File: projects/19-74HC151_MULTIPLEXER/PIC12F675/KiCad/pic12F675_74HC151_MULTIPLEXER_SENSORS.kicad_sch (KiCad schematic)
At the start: 13 parts, among them M1 Motor_DC, M2 Motor_DC, Q1 NMOS, Q2 NMOS, U1 PIC12F675-IP, U2 74151, U3 LM35-LP, U4 A1369xUA-10, U5 LM35-LP, U6 A1369xUA-10

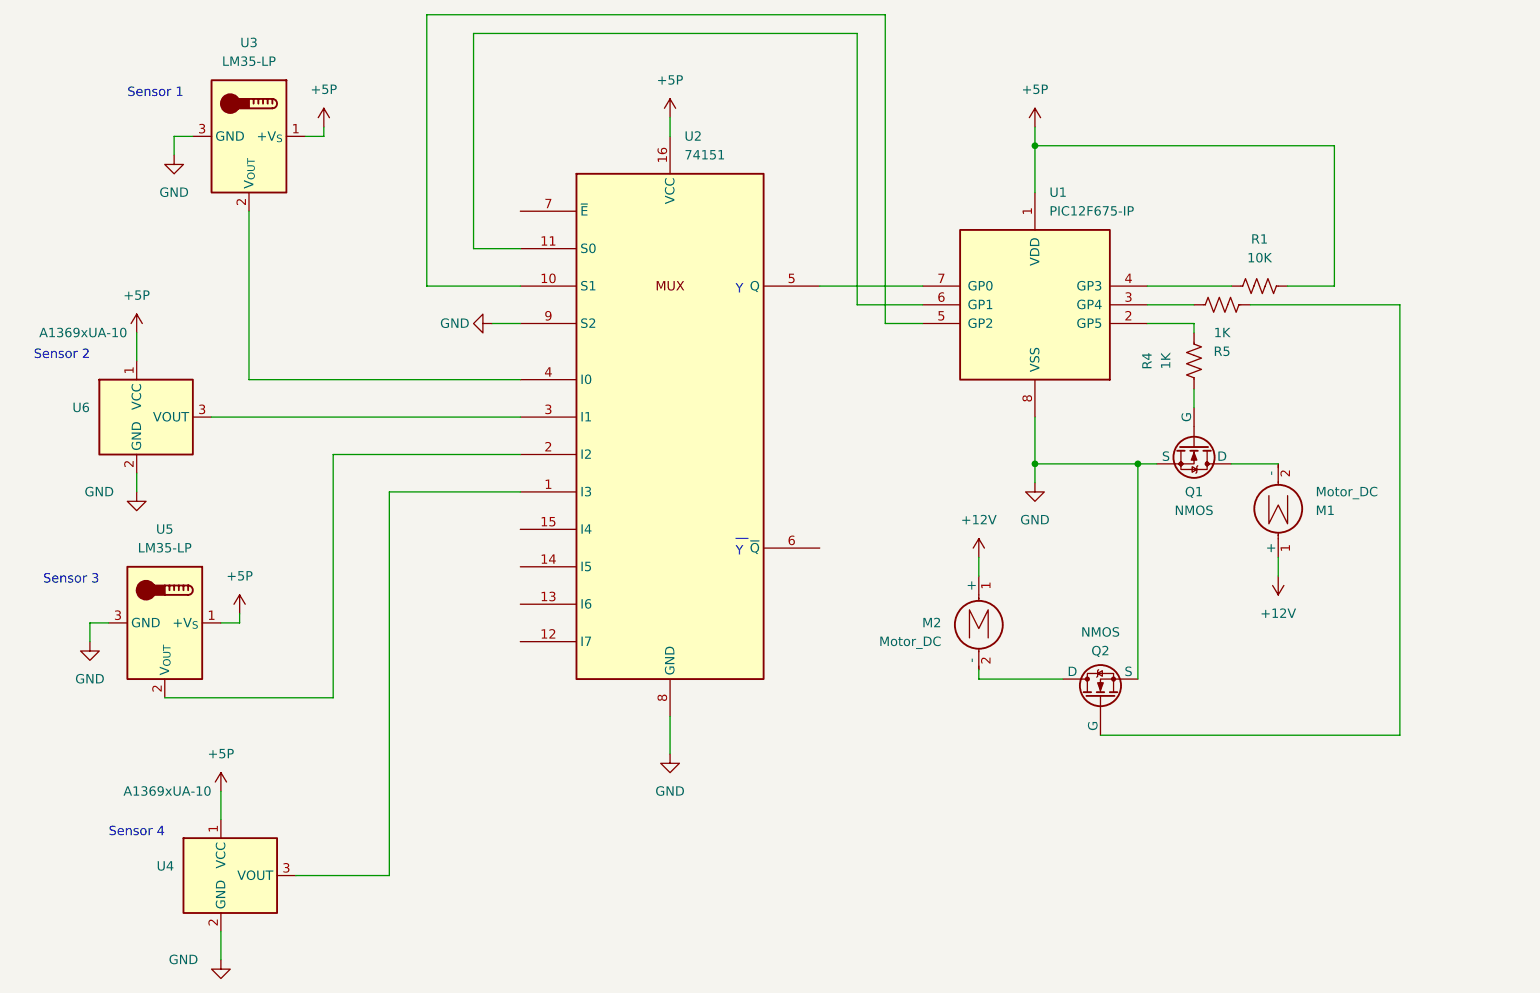
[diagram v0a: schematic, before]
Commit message: Doc
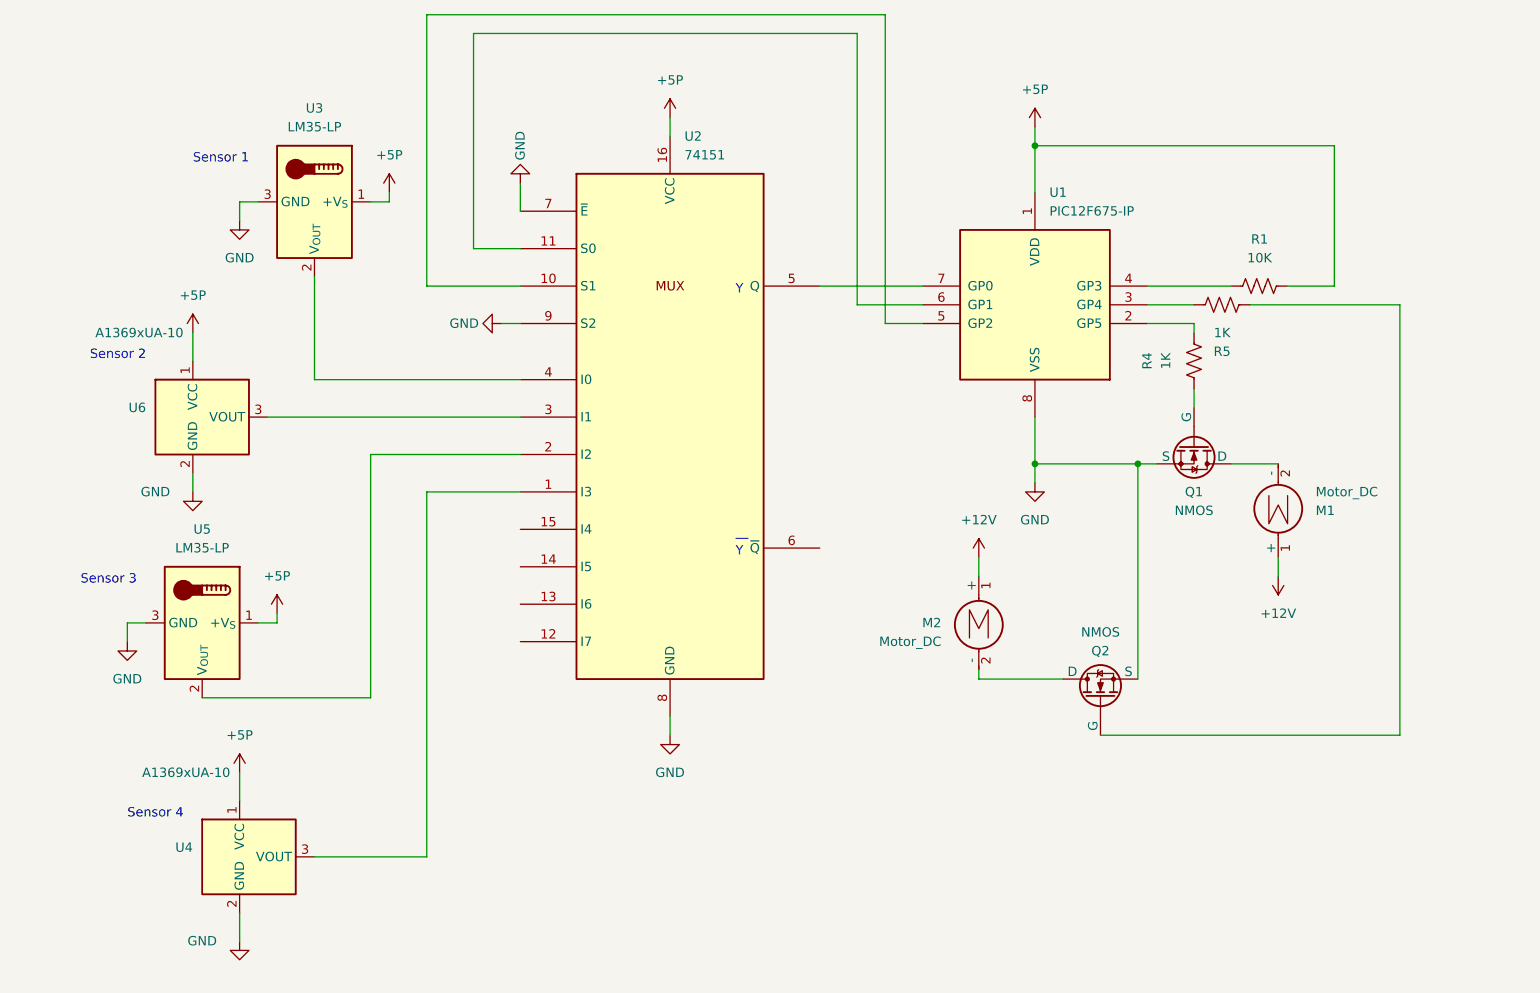
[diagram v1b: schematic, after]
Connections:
- net GND: now also U2.7 (~{E})
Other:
- moved on the sheet: U3, U4, U5, U6

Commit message: Doc
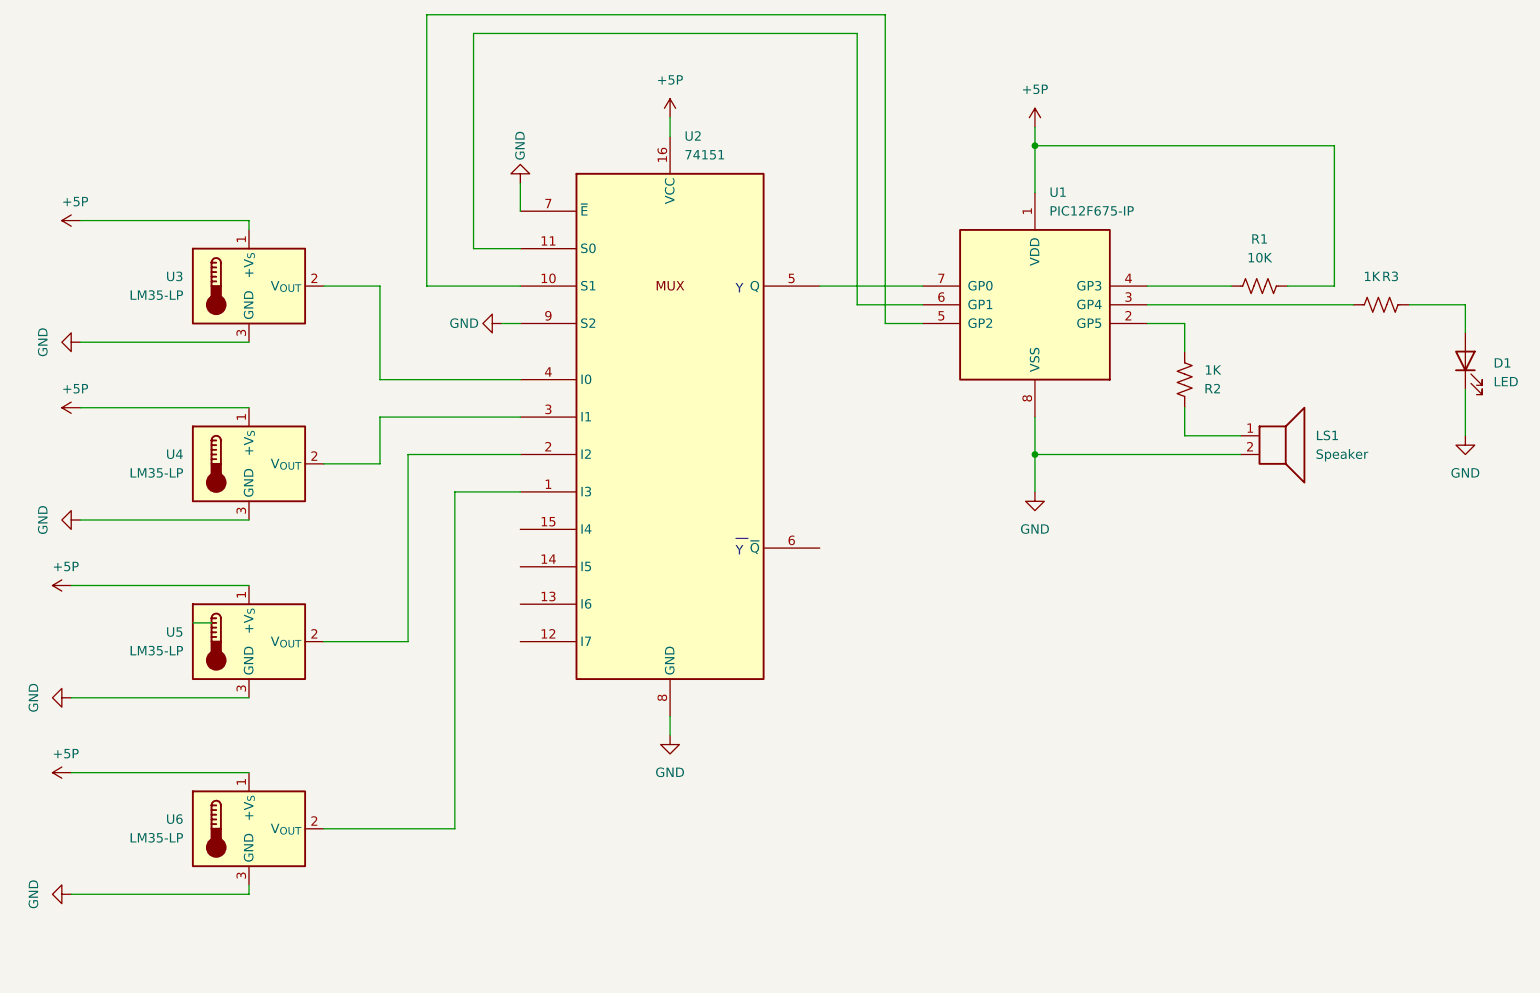
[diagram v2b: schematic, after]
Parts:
- removed M1, M2: Motor_DC, symbol Motor:Motor_DC
- removed Q1, Q2: NMOS, symbol Simulation_SPICE:NMOS
- removed R4, R5: 1K, symbol Device:R_US
- removed U4, U6: A1369xUA-10, Sensor_Current:Allegro_SIP-3, symbol Sensor_Current:A1369xUA-10
- added D1: LED, symbol Device:LED
- added LS1: Speaker, symbol Device:Speaker
- added R2, R3: 1K, symbol Device:R_US
- added U4, U6: LM35-LP, Package_TO_SOT_THT:TO-92_Inline, symbol Sensor_Temperature:LM35-LP
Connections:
- net +5P: now also U4.1 (+V_{S}), U6.1 (+V_{S})
- net GND: now also D1.1 (K), LS1.2, U4.3 (GND), U6.3 (GND)
- net at U1.3 (GP4): now also R3.1
- net at U2.1 (I3): now also U6.2 (V_{OUT})
- net at U2.3 (I1): now also U4.2 (V_{OUT})
- net at U1.2 (GP5): now also R2.1
- new net: LS1.1, R2.2
- new net: D1.2 (A), R3.2
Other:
- note removed: "Sensor 1"
- note removed: "Sensor 2"
- note removed: "Sensor 3"
- note removed: "Sensor 4"
- moved on the sheet: U3, U5

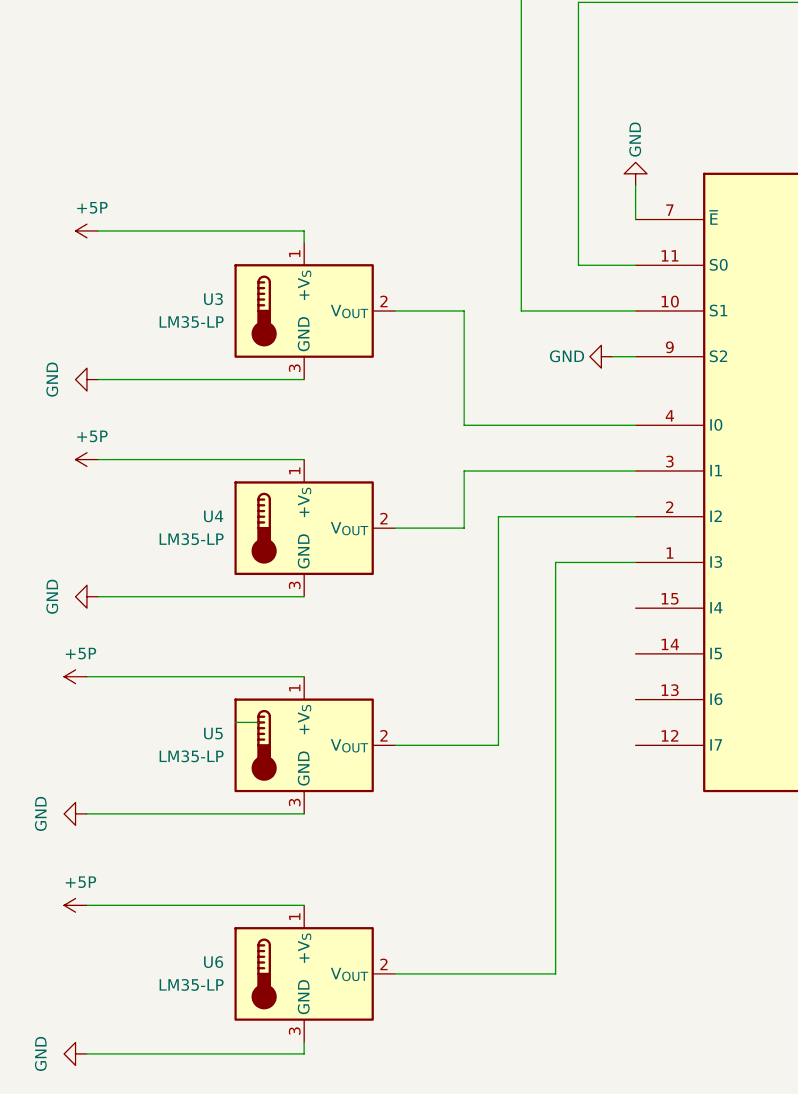
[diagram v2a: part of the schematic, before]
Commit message: Doc
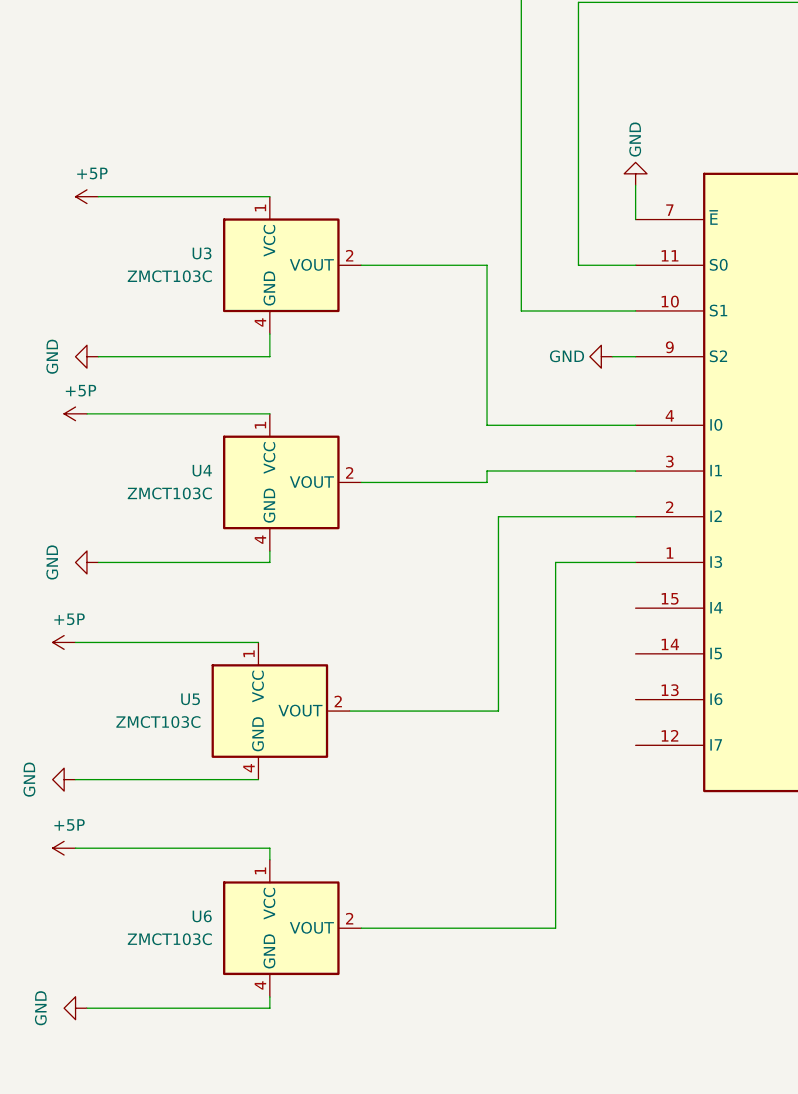
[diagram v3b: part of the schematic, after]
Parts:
- removed U3, U4, U5, U6: LM35-LP, Package_TO_SOT_THT:TO-92_Inline, symbol Sensor_Temperature:LM35-LP
- added U3, U4, U5, U6: ZMCT103C, Sensor_Current:Allegro_SIP-4, symbol Sensor_Current:A1363xKTTN-1
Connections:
- net +5P: now also U3.1 (VCC), U4.1 (VCC), U5.1 (VCC), U6.1 (VCC)
- net GND: now also U3.4 (GND), U4.4 (GND), U5.4 (GND), U6.4 (GND)
- net at U2.3 (I1): now also U4.2 (VOUT)
- net at U2.1 (I3): now also U6.2 (VOUT)
- net at U2.2 (I2): now also U5.2 (VOUT)
- net at U2.4 (I0): now also U3.2 (VOUT)
